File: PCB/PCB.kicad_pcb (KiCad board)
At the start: 2 copper layers, 11 parts

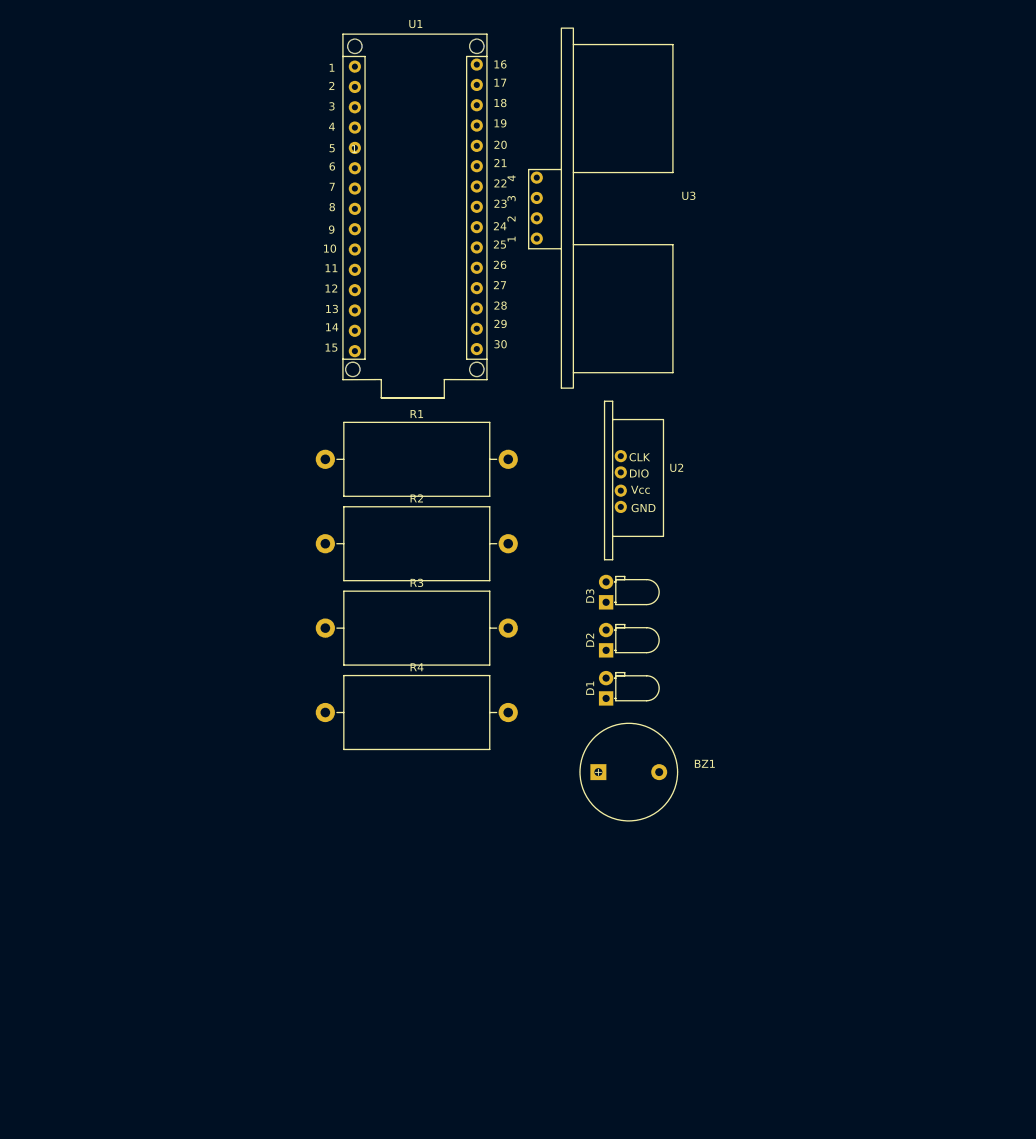
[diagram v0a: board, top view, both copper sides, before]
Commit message: Routing & DRC of PCB
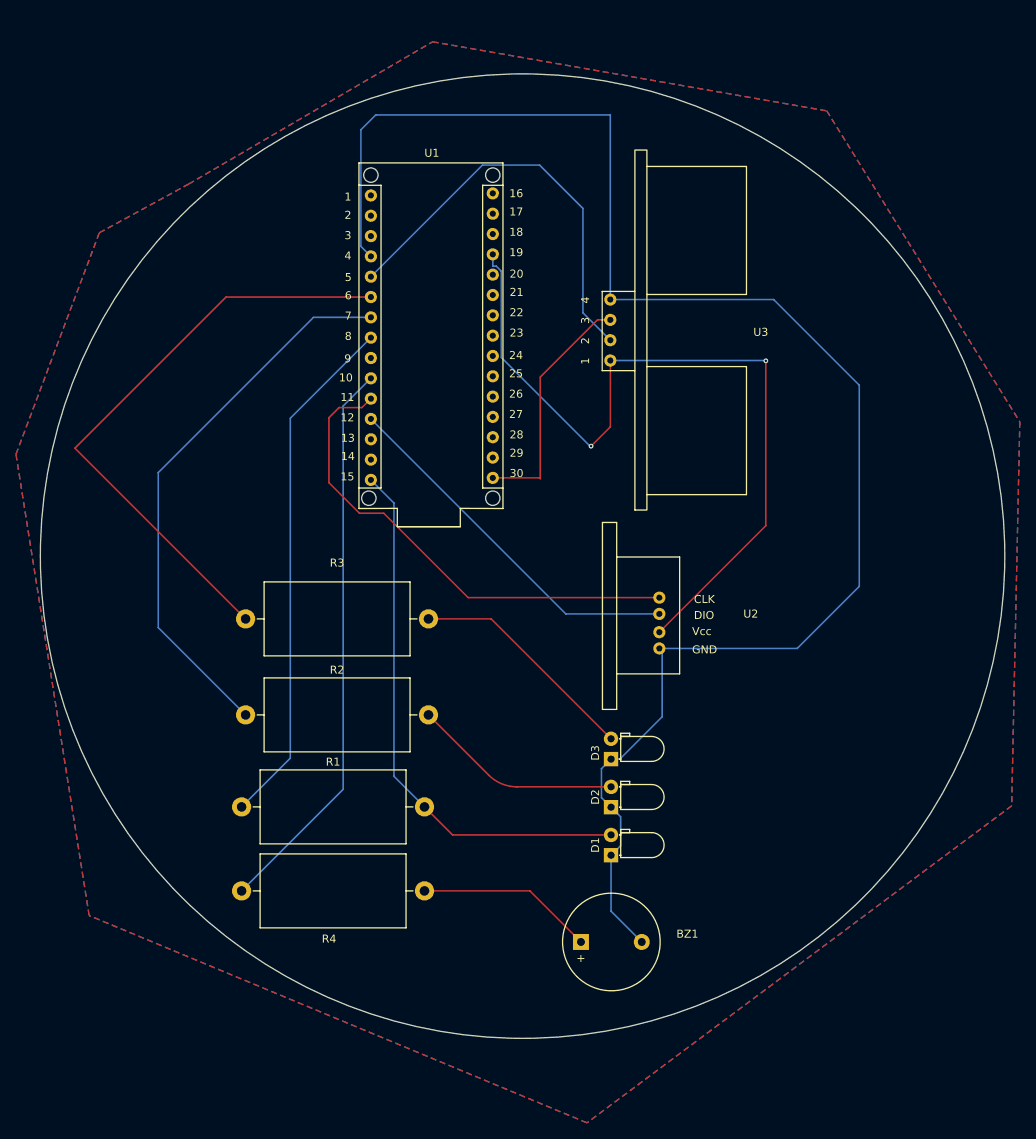
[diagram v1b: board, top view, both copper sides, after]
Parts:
- moved R1 44.7 mm to (117.1, 124.8)
- moved R4 24.6 mm to (117.1, 135.3)
- moved R2 23.6 mm to (117.6, 113.3)
- moved BZ1 21.3 mm to (159.5, 141.7)
- moved D2 19.6 mm to (163.3, 124.9)
- moved D3 19.6 mm to (163.3, 118.9)
- moved D1 19.6 mm to (163.3, 130.9)
- moved U3 17.8 mm to (167.0, 65.2)
- moved U2 17.2 mm to (163.5, 101.5)
- moved U1 16.2 mm to (140.4, 65.9)
- moved R3 10.0 mm to (117.6, 101.3)
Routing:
- net GND: track 0.00 -> 204.0 mm
- net Source: track 0.00 -> 99.8 mm, vias 0 -> 2
- net GREEN: track 0.00 -> 75.0 mm
- net Buzz: track 0.00 -> 70.8 mm
- net YELLOW: track 0.00 -> 69.4 mm
- net REDR: track 0.00 -> 68.4 mm
- net RED: track 0.00 -> 65.3 mm
- net CLK: track 0.00 -> 61.6 mm
- net Trigger: track 0.00 -> 52.4 mm
- net DIO: track 0.00 -> 46.2 mm
- net Echo: track 0.00 -> 30.4 mm
- net Net-(D3-A): track 0.00 -> 29.6 mm
- net Net-(D2-A): track 0.00 -> 26.3 mm
- net Net-(BZ1-+): track 0.00 -> 22.2 mm
- added copper zone on B.Cu, net GND
- added copper zone on F.Cu, net GND
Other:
- board outline added: 120.6 x 120.6 mm
